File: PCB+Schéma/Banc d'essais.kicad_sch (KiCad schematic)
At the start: 6 parts, among them U1 MCP4431-xxxx-ST

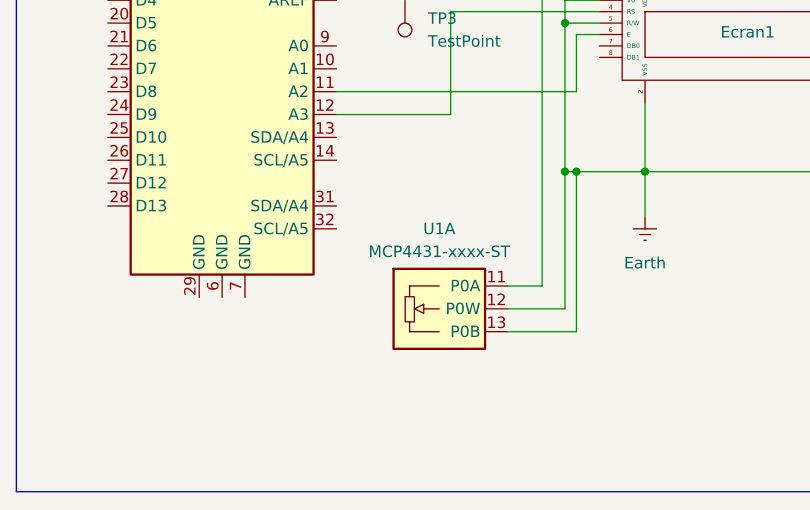
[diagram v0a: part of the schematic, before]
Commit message: mise a jours
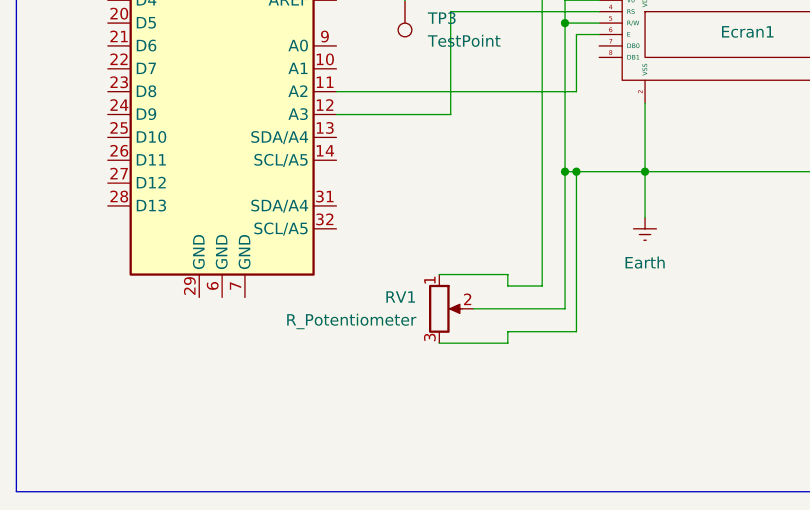
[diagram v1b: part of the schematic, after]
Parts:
- removed U1: MCP4431-xxxx-ST, Package_SO:TSSOP-20_4.4x6.5mm_P0.65mm, symbol Potentiometer_Digital:MCP4431-xxxx-ST
- added RV1: R_Potentiometer, Potentiometer_THT:Potentiometer_ACP_CA6-H2,5_Horizontal, symbol Device:R_Potentiometer
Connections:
- net Earth: now also RV1.2, RV1.3
- net at A1.3 (~{RESET}), A1.4 (3V3), A1.5 (+5V)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: now also RV1.1
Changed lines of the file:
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@@
+	(wire
+		(pts
+			(xy 134.62 109.22) (xy 142.24 109.22)
+		)
+		(stroke
+			(width 0)
+			(type default)
+		)
+	)
 	(wire
 		(pts
@@
 	(wire
 		(pts
+			(xy 142.24 109.22) (xy 142.24 110.49)
+		)
+		(stroke
+			(width 0)
+			(type default)
+		)
+	)
+	(wire
+		(pts
 			(xy 146.05 71.12) (xy 157.48 71.12)
 		)
@@
 	(wire
 		(pts
-			(xy 148.59 113.03) (xy 142.24 113.03)
+			(xy 138.43 113.03) (xy 148.59 113.03)
 		)
 		(stroke
@@
 	(wire
 		(pts
+			(xy 134.62 116.84) (xy 142.24 116.84)
+		)
+		(stroke
+			(width 0)
+			(type default)
+		)
+	)
+	(wire
+		(pts
 			(xy 148.59 97.79) (xy 149.86 97.79)
 		)
@@
 	(wire
 		(pts
+			(xy 142.24 116.84) (xy 142.24 115.57)
+		)
+		(stroke
+			(width 0)
+			(type default)
+		)
+	)
+	(wire
+		(pts
 			(xy 148.59 97.79) (xy 148.59 113.03)
 		)
@@
 			(width 0)
 			(type default)
+		)
+	)
+	(symbol
+		(lib_id "Device:R_Potentiometer")
+		(at 134.62 113.03 0)
+		(unit 1)
+		(exclude_from_sim no)
+		(in_bom yes)
+		(on_board yes)
+		(dnp no)
+		(fields_autoplaced yes)
+		(property "Reference" "RV1"
+			(at 132.08 111.7599 0)
+			(effects
+				(font
+					(size 1.27 1.27)
+				)
+				(justify right)
+			)
+		)
+		(property "Value" "R_Potentiometer"
+			(at 132.08 114.2999 0)
+			(effects
+				(font
+					(size 1.27 1.27)
+				)
+				(justify right)
+			)
+		)
+		(property "Footprint" "Potentiometer_THT:Potentiometer_ACP_CA6-H2,5_Horizontal"
+			(at 134.62 113.03 0)
+			(effects
+				(font
+					(size 1.27 1.27)
+				)
+				(hide yes)
+			)
+		)
+		(property "Datasheet" "~"
+			(at 134.62 113.03 0)
+			(effects
+				(font
+					(size 1.27 1.27)
+				)
+				(hide yes)
+			)
+		)
+		(property "Description" "Potentiometer"
+			(at 134.62 113.03 0)
+			(effects
+				(font
+					(size 1.27 1.27)
+				)
+				(hide yes)
+			)
+		)
+		(pin "3"
+		)
+		(pin "2"
+		)
+		(pin "1"
+		)
+		(instances
+			(project ""
+				(path "/137ff572-d30e-44d7-a0ef-739ddc99a077"
+					(reference "RV1")
+					(unit 1)
+				)
+			)
 		)
 	)
@@
 					(unit 1)
 				)
-			)
-		)
-	)
-	(symbol
-		(lib_id "Potentiometer_Digital:MCP4431-xxxx-ST")
-		(at 134.62 113.03 180)
-		(unit 1)
-		(exclude_from_sim no)
-		(in_bom yes)
-		(on_board yes)
-		(dnp no)
-		(fields_autoplaced yes)
-		(property "Reference" "U1"
-			(at 134.62 104.14 0)
-			(effects
-				(font
-					(size 1.27 1.27)
-				)
-			)
-		)
-		(property "Value" "MCP4431-xxxx-ST"
-			(at 134.62 106.68 0)
-			(effects
-				(font
-					(size 1.27 1.27)
-				)
-			)
-		)
-		(property "Footprint" "Package_SO:TSSOP-20_4.4x6.5mm_P0.65mm"
-			(at 134.62 100.33 0)
-			(effects
-				(font
-					(size 1.27 1.27)
-				)
-				(hide yes)
-			)
-		)
-		(property "Datasheet" "https://ww1.microchip.com/downloads/en/DeviceDoc/22267A_MCP4431.pdf"
-			(at 134.62 97.79 0)
-			(effects
-				(font
-					(size 1.27 1.27)
-				)
-				(hide yes)
-			)
-		)
-		(property "Description" "Quad 7 Bit Digital Potentiometer, I²C, Volatile Memory, TSSOP-20"
-			(at 134.62 113.03 0)
-			(effects
-				(font
-					(size 1.27 1.27)
-				)
-				(hide yes)
-			)
-		)
-		(pin "12"
-		)
-		(pin "10"
-		)
-		(pin "2"
-		)
-		(pin "9"
-		)
-		(pin "14"
-		)
-		(pin "20"
-		)
-		(pin "18"
-		)
-		(pin "1"
-		)
-		(pin "5"
-		)
-		(pin "16"
-		)
-		(pin "13"
-		)
-		(pin "11"
-		)
-		(pin "6"
-		)
-		(pin "3"
-		)
-		(pin "19"
-		)
-		(pin "17"
-		)
-		(pin "7"
-		)
-		(pin "8"
-		)
-		(pin "15"
-		)
-		(pin "4"
-		)
-		(instances
-			(project "Banc d'essais"
-				(path "/137ff572-d30e-44d7-a0ef-739ddc99a077"
-					(reference "U1")
-					(unit 1)
-				)
